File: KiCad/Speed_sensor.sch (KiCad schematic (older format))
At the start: 69 parts, among them J1 USB_B_Micro, J2 SWD, U1 BQ24040DSQR, U2 TP1941U, U3 ST1PS02, U4 nRF52832-QFxx, U5 LIS2DH12, Y1 32,768kHz, Y2 32MHz

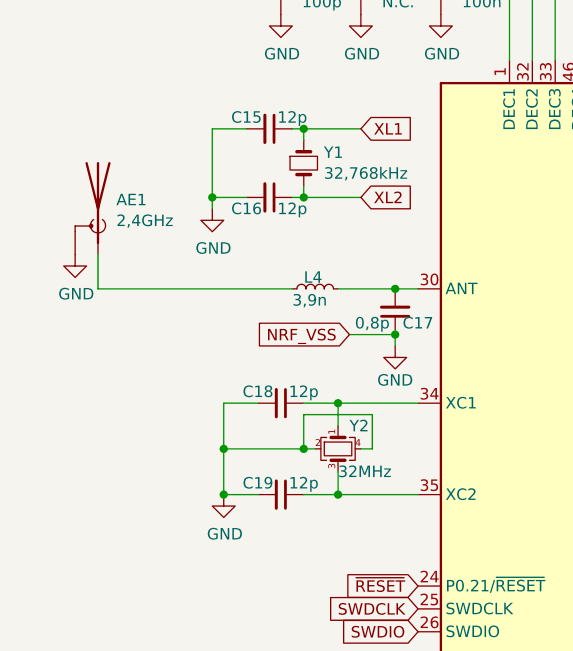
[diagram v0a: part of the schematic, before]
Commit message: small changes in the layout
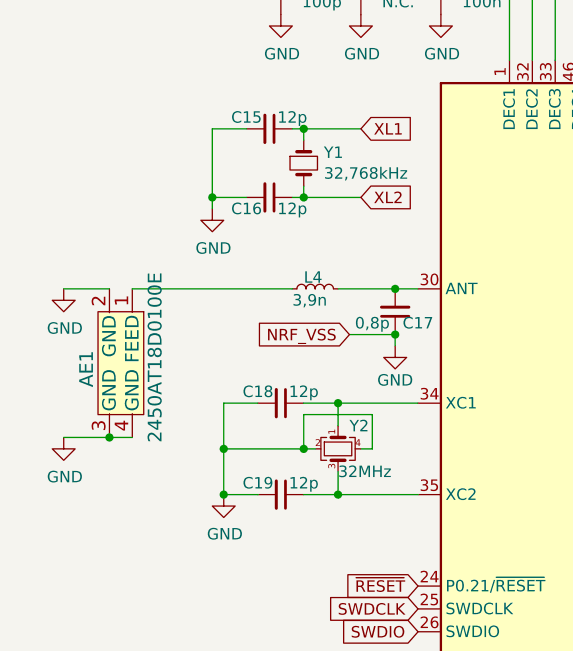
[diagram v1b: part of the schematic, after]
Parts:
- removed AE1: 2,4GHz, RF_Antenna:Texas_SWRA117D_2.4GHz_Right, symbol Device:Antenna_Shield
- added AE1: 2450AT18D0100E, myparts:2450AT18D0100E, symbol myparts:2450AT18D0100E
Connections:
- net GND: now also AE1.2 (GND), AE1.3 (GND), AE1.4 (GND)
- net at L4.1: now also AE1.1 (FEED)
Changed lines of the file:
@@
 Wire Wire Line
 	1750 5700 2050 5700
-Wire Wire Line
-	850  5000 850  5150
-Wire Wire Line
-	850  5150 1700 5150
 Text Notes 10550 1800 0    25   ~ 0
 R10 kann evtl. entfernt werden.
-$Comp
-L Device:Antenna_Shield AE1
-U 1 1 608E3518
-P 850 4800
-F 0 "AE1" H 770 4839 50  0000 R CNN
-F 1 "2,4GHz" H 770 4748 50  0000 R CNN
-F 2 "RF_Antenna:Texas_SWRA117D_2.4GHz_Right" H 850 4900 50  0001 C CNN
-F 3 "~" H 850 4900 50  0001 C CNN
-	1    850  4800
-	-1   0    0    -1
-$EndComp
-$Comp
-L power:GND #PWR035
-U 1 1 608ED256
-P 750 5000
-F 0 "#PWR035" H 750 4750 50  0001 C CNN
-F 1 "GND" H 755 4827 50  0000 C CNN
-F 2 "" H 750 5000 50  0001 C CNN
-F 3 "" H 750 5000 50  0001 C CNN
-	1    750  5000
-	1    0    0    -1
-$EndComp
 $Comp
 L Device:C_Small C5
@@
 Wire Wire Line
 	6200 4550 6350 4550
+$Comp
+L myparts:2450AT18D0100E AE1
+U 1 1 6099F4A4
+P 1000 5450
+F 0 "AE1" H 1050 5250 60  0000 C CNN
+F 1 "2450AT18D0100E" H 1000 5550 60  0000 C CNN
+F 2 "myparts:2450AT18D0100E" H 1150 5400 60  0001 C CNN
+F 3 "" H 1300 5450 60  0001 C CNN
+	1    1000 5450
+	0    1    1    0
+$EndComp
+Wire Wire Line
+	1000 5150 1700 5150
+$Comp
+L power:GND #PWR035
+U 1 1 609D15A8
+P 700 5150
+F 0 "#PWR035" H 700 4900 50  0001 C CNN
+F 1 "GND" H 705 4977 50  0000 C CNN
+F 2 "" H 700 5150 50  0001 C CNN
+F 3 "" H 700 5150 50  0001 C CNN
+	1    700  5150
+	1    0    0    -1
+$EndComp
+Wire Wire Line
+	700  5150 900  5150
+$Comp
+L power:GND #PWR036
+U 1 1 609D8BDF
+P 700 5800
+F 0 "#PWR036" H 700 5550 50  0001 C CNN
+F 1 "GND" H 705 5627 50  0000 C CNN
+F 2 "" H 700 5800 50  0001 C CNN
+F 3 "" H 700 5800 50  0001 C CNN
+	1    700  5800
+	1    0    0    -1
+$EndComp
+Wire Wire Line
+	1000 5800 900  5800
+Connection ~ 900  5800
+Wire Wire Line
+	900  5800 700  5800
 $EndSCHEMATC

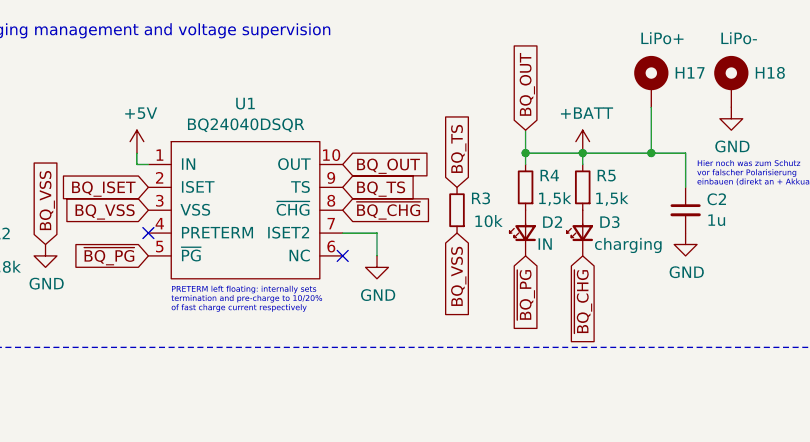
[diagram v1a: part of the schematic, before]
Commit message: layout part placement (again, very small changes)
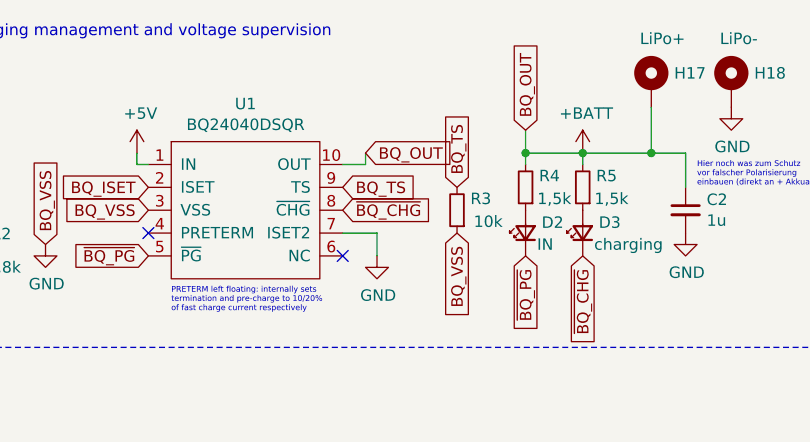
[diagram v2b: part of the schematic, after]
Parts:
- Y1: footprint myparts:TestPoint_2Pads_Pitch1mm_Drill0.4mm -> Crystal:Crystal_SMD_G8-2Pin_3.2x1.5mm
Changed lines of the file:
@@
 	1    0    0    -1
 $EndComp
-Text GLabel 4000 1150 2    50   Input ~ 0
+Text GLabel 4100 1100 2    50   Input ~ 0
 BQ_OUT
 Text GLabel 4000 1250 2    50   Input ~ 0
@@
 F 0 "Y1" V 1704 4688 50  0000 L CNN
 F 1 "32,768kHz" V 1795 4688 50  0000 L CNN
-F 2 "myparts:TestPoint_2Pads_Pitch1mm_Drill0.4mm" H 1750 4600 50  0001 C CNN
+F 2 "Crystal:Crystal_SMD_G8-2Pin_3.2x1.5mm" H 1750 4600 50  0001 C CNN
 F 3 "~" H 1750 4600 50  0001 C CNN
 	1    1750 4600
@@
 Wire Wire Line
 	900  5800 700  5800
+Wire Wire Line
+	4100 1100 4100 1150
+Wire Wire Line
+	4100 1150 4000 1150
 $EndSCHEMATC
